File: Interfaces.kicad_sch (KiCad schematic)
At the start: 4 parts, among them J4 Conn_01x40_Socket, J5 Conn_01x05_Pin, J6 Conn_01x05_Pin, J9 Conn_01x02_Pin

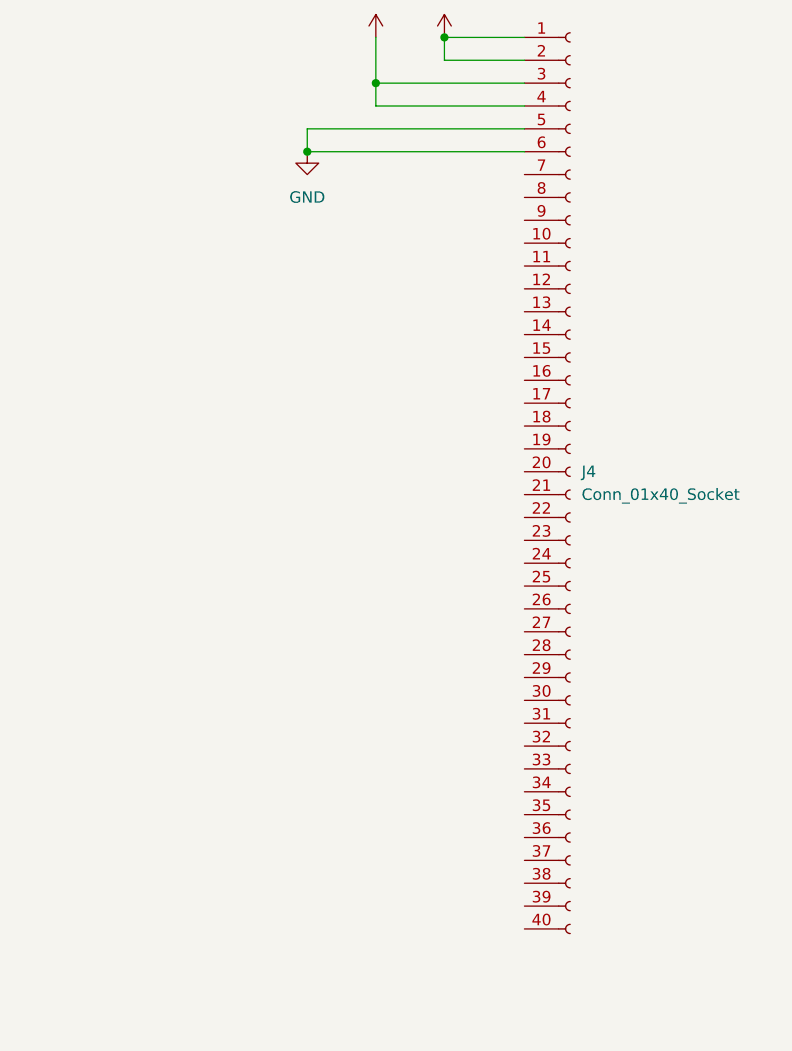
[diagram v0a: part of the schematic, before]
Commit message: completed layout and routing
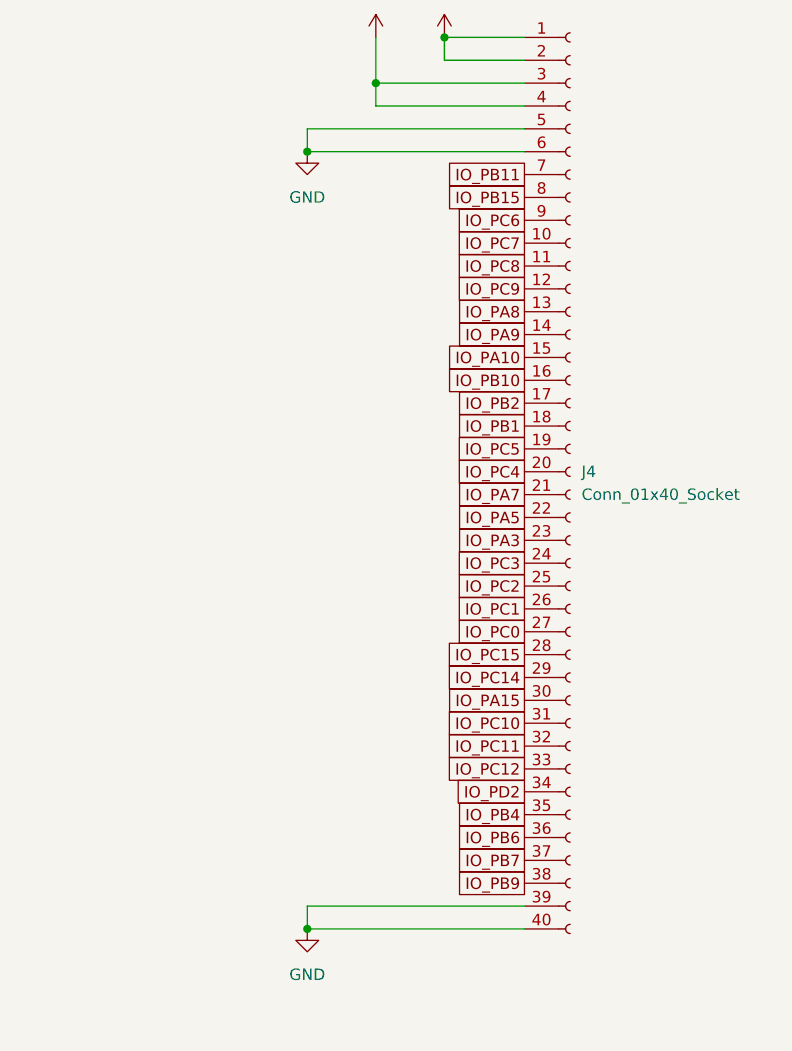
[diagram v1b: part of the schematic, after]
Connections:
- net GND: now also J4.39 (Pin_39), J4.40 (Pin_40)
- net IO_PC7: now reaches J4.10 (Pin_10)
- net IO_PC8: now reaches J4.11 (Pin_11)
- net IO_PC9: now reaches J4.12 (Pin_12)
- net IO_PA8: now reaches J4.13 (Pin_13)
- net IO_PA9: now reaches J4.14 (Pin_14)
- net IO_PA10: now reaches J4.15 (Pin_15)
- net IO_PB10: now reaches J4.16 (Pin_16)
- net IO_PB2: now reaches J4.17 (Pin_17)
- net IO_PB1: now reaches J4.18 (Pin_18)
- net IO_PC5: now reaches J4.19 (Pin_19)
- net IO_PC4: now reaches J4.20 (Pin_20)
- net IO_PA7: now reaches J4.21 (Pin_21)
- net IO_PA5: now reaches J4.22 (Pin_22)
- net IO_PA3: now reaches J4.23 (Pin_23)
- net IO_PC3: now reaches J4.24 (Pin_24)
- net IO_PC2: now reaches J4.25 (Pin_25)
- net IO_PC1: now reaches J4.26 (Pin_26)
- net IO_PC0: now reaches J4.27 (Pin_27)
- net IO_PC15: now reaches J4.28 (Pin_28)
- net IO_PC14: now reaches J4.29 (Pin_29)
- net IO_PA15: now reaches J4.30 (Pin_30)
- net IO_PC10: now reaches J4.31 (Pin_31)
- net IO_PC11: now reaches J4.32 (Pin_32)
- net IO_PC12: now reaches J4.33 (Pin_33)
- net IO_PD2: now reaches J4.34 (Pin_34)
- net IO_PB4: now reaches J4.35 (Pin_35)
- net IO_PB6: now reaches J4.36 (Pin_36)
- net IO_PB7: now reaches J4.37 (Pin_37)
- net IO_PB9: now reaches J4.38 (Pin_38)
- net IO_PB11: now reaches J4.7 (Pin_7)
- net IO_PB15: now reaches J4.8 (Pin_8)
- net IO_PC6: now reaches J4.9 (Pin_9)
